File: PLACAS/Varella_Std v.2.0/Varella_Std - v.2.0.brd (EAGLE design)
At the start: 86 x 86 mm, 92 parts, among them IC1 74HC4051D,653, IC3 M95M04-DRDW6TP, IC4 M95M04-DRDW6TP, IC5 M95M04-DRDW6TP, IC6 M95M04-DRDW6TP, IC7 TESEO-LIV3F, IC8 BGA_725L6_E6327, U1 MAX31856, U2 MAX31856, U3 MAX31856, X1 JST-XH-02-PIN-ROUND-PAD, X2 JST-XH-02-PIN-ROUND-PAD, X3 JST-XH-02-PIN-ROUND-PAD

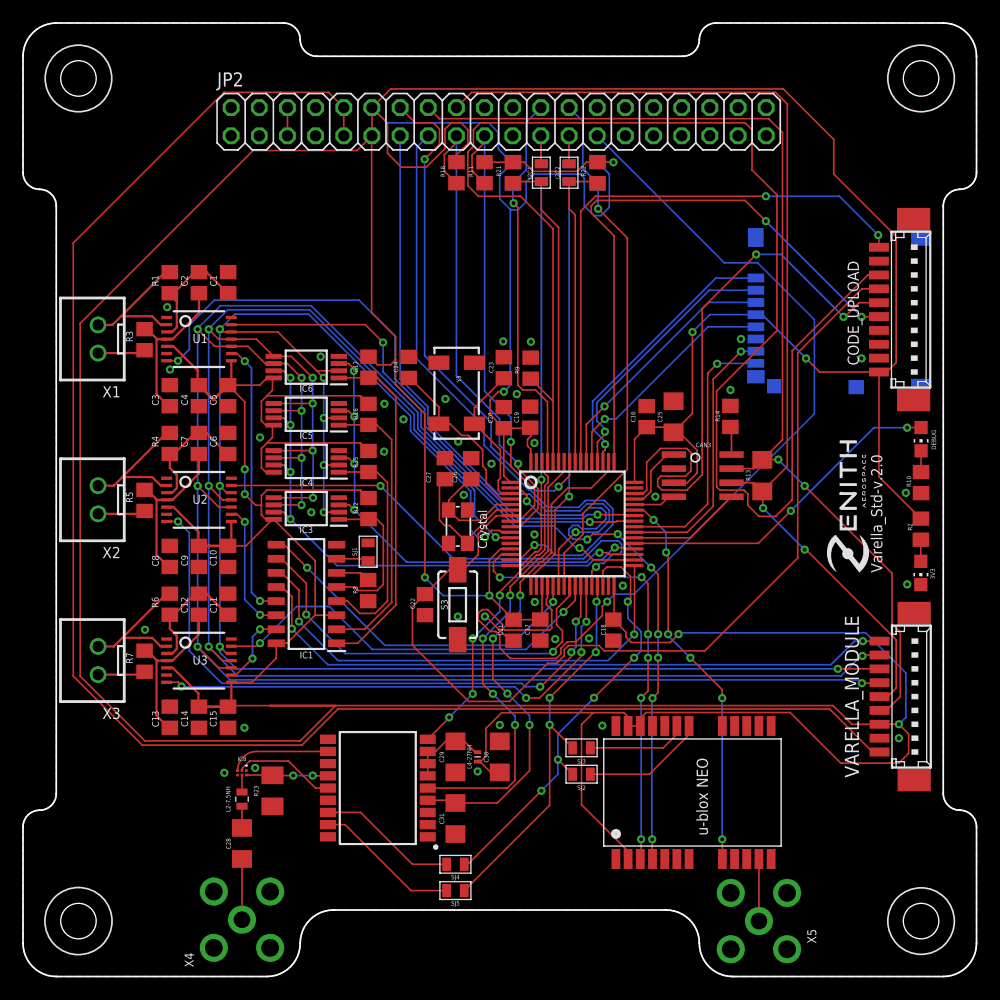
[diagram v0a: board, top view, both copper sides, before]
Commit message: Add files via upload
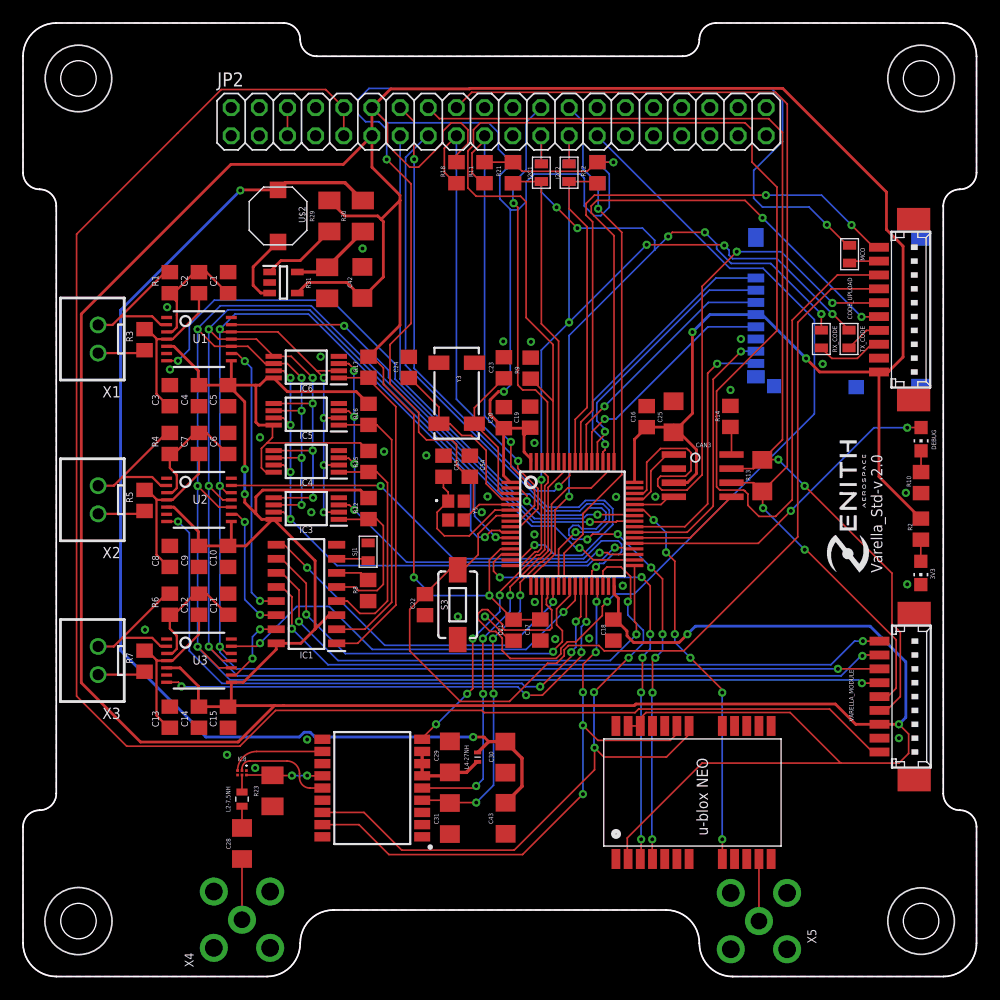
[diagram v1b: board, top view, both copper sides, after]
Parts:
- removed C26, C27: (no value), rcl:C0805
- removed SJ2, SJ3, SJ4, SJ5: (no value), FaBo-PIN:SMD-JUMPER-2
- removed U$7: CRYSTAL, cristal:CRYSTAL_SMD
- added C42: 56pF, rcl:C1206
- added C43: 22uF, rcl:C1206
- added C54, C55: 10pF, rcl:C0805
- added IC13: ST1S12GR, SamacSys_Parts:SOT95P280X110-5N
- added MCO, RX_CODE, TX_CODE: (no value), FaBo-PIN:SMD-JUMPER-2
- added R29: 1M, rcl (2):M1206
- added R30: 68k, rcl (2):M1206
- added R31: 27k, rcl (2):M1206
- added U$2: LTF5022T100M1R4, LTF5022T:LTF5022T
- added Y5: FA-20H_16.0000MF10Z-AJ0, SamacSys_Parts:FA20H160000MF12ZAC3
- C16, C17, C18, C19, C20: value (none) -> 100nF
- C21: value (none) -> 1uF
- C22: value (none) -> 0,1uF
- C23, C24: value (none) -> 10pF
- R10: value (none) -> 220
- R11, R12, R15, R16, R17, R18, R19, R20, R21, R22: value (none) -> 4,7k
- R8, R9: value (none) -> 1k
- moved C30 0.50 mm to (43.5, 19.8), turned to 270 degrees
- moved C29 0.50 mm to (38.5, 19.8), turned to 90 degrees
- moved C31 0.50 mm to (38.5, 14.2)
- moved IC7 0.50 mm to (31.5, 17.0)
- turned L4-27NH to 270 degrees
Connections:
- net SDA1/UART_TX renamed SDA1/UART_RX
- net SDA2/UART_RX renamed SDA2/UART_TX
- removed net SCL_NEOM8: SJ3.1, U$3.19
- removed net SCL_TESEO: IC7.17, SJ5.1
- removed net SDA_NEOM8: SJ2.1, U$3.18
- removed net SDA_TESEO: IC7.16, SJ4.1
- new net N$37: IC13.1, R29.1
- new net N$38: IC13.3, U$2.P$2
- new net N$39: IC13.5, R30.1, R31.2
- new net TESEO3: C30.1, C43.1, L4-27NH.1, R30.2, U$2.P$1
- new net UART_RX_CODE: CODE_UPLOAD.3, RX_CODE.2
- new net UART_TX_CODE: CODE_UPLOAD.4, TX_CODE.2
- net +3V3: now also C42.1, IC13.4, R29.2; no longer C30.1, L4-27NH.1
- net GND: now also C42.2, C43.2, C54.2, C55.2, IC13.2, R31.1, Y5.2, Y5.4; no longer C26.2, C27.2, U$7.P$1, U$7.P$4
- net MCO: now also MCO.2
- net OSC_IN: now also C54.1, MCO.1, Y5.3; no longer C26.1, U$7.P$2
- net OSC_OUT: now also C55.1, Y5.1; no longer C27.1, U$7.P$3
- net SCL4: now also IC7.17, U$3.19; no longer SJ3.2, SJ5.2
- net SDA4: now also IC7.16, U$3.18; no longer SJ2.2, SJ4.2
- net UART_RX: now also RX_CODE.1, UART_TX.2; no longer UART_RX.2
- net UART_TX: now also TX_CODE.1, UART_RX.2; no longer UART_TX.2
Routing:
- net TESEO3: track 0.00 -> 104.7 mm, vias 0 -> 2
- net OSC_IN: track 11.2 -> 110.4 mm, vias 0 -> 2
- net UART_TX: track 36.5 -> 69.1 mm, vias 1 -> 5
- net UART_RX: track 38.0 -> 69.3 mm, vias 1 -> 6
- net SDA4: track 39.6 -> 64.6 mm, vias 5 -> 4
- net SCL4: track 36.1 -> 57.7 mm, vias 4 -> 5
- net SCL_TESEO: track 13.2 -> 0.00 mm
- net SDA_TESEO: track 12.6 -> 0.00 mm
- net +3V3: track 683.8 -> 695.6 mm
- net SDA_NEOM8: track 11.2 -> 0.00 mm
- net SCL_NEOM8: track 9.08 -> 0.00 mm
- net N$39: track 0.00 -> 7.55 mm
- net N$37: track 0.00 -> 6.90 mm
- net N$38: track 0.00 -> 6.61 mm
- net UART_RX_CODE: track 0.00 -> 6.12 mm
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
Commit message: Add files via upload
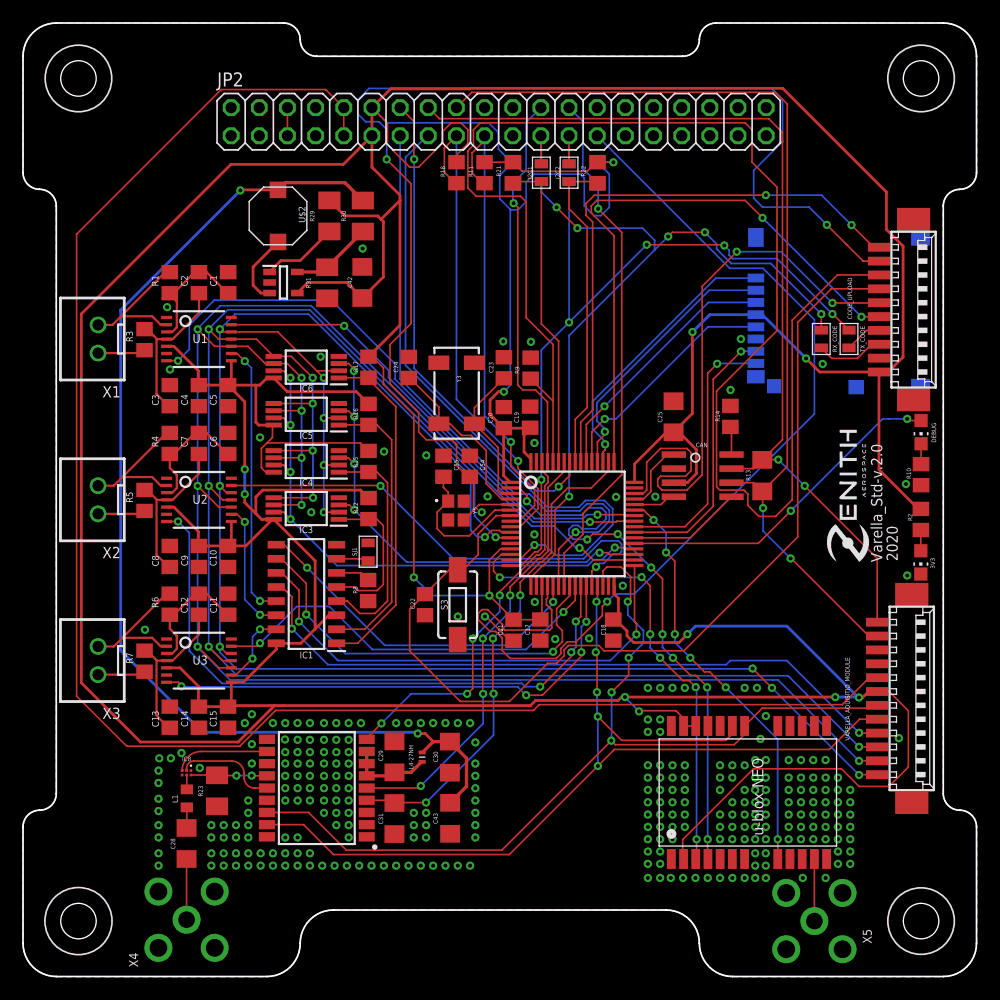
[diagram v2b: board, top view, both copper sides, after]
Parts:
- removed C16: 100nF, rcl:C0805
- removed L2-7,5NH: 0603CS-7N5XGLU, SamacSys_Parts:0603CS82NXGLW
- removed MCO: (no value), FaBo-PIN:SMD-JUMPER-2
- removed VARELLA_MODULE: 53398-09, con-molex:53398-09
- added L1: LQW18AS7N5J0ZD-7,5nH, LQW18AS7N5J0ZD:INDC1608X100N
- added VARELLA_AQUISITIO_MODULE: 53261-12, con-molex:53261-12
- CODE_UPLOAD: value 53398-10 -> 53261-10; device con-molex:53398-10 -> con-molex:53261-10
- moved C28 5.00 mm to (14.8, 12.0)
- moved C29 5.00 mm to (33.5, 19.8)
- moved C30 5.00 mm to (38.5, 19.8)
- moved C31 5.00 mm to (33.5, 14.2)
- moved C43 5.00 mm to (38.5, 14.3)
- moved IC7 5.00 mm to (26.5, 17.0)
- moved IC8 5.00 mm to (14.8, 18.4)
- moved L4-27NH 5.00 mm to (36.0, 19.8)
- moved R23 5.00 mm to (17.5, 16.8)
- moved U$3 5.00 mm to (65.9, 17.0)
- moved X4 5.00 mm to (14.8, 5.12)
- moved X5 5.00 mm to (71.4, 5.00)
- moved 3V3 0.95 mm to (81.0, 37.4)
- moved R2 0.87 mm to (81.0, 41.2)
- moved R10 0.71 mm to (81.0, 45.3)
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- renumbered CAN3 to CAN, COMM_MICRO1 to COMM_MICRO
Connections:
- net N$2 renamed L3
- removed net MCO: CODE_UPLOAD.9, MCO.2
- net +3V3: now also VARELLA_AQUISITIO_MODULE.7; no longer C16.1, VARELLA_MODULE.3
- net +5V: now also VARELLA_AQUISITIO_MODULE.8; no longer VARELLA_MODULE.1
- net CAN_H: now also VARELLA_AQUISITIO_MODULE.12; no longer VARELLA_MODULE.4
- net CAN_L: now also VARELLA_AQUISITIO_MODULE.11; no longer VARELLA_MODULE.5
- net GND: now also VARELLA_AQUISITIO_MODULE.10, VARELLA_AQUISITIO_MODULE.9; no longer C16.2, VARELLA_MODULE.2
- net MISO_SENSOR: now also VARELLA_AQUISITIO_MODULE.1; no longer VARELLA_MODULE.7
- net MOSI_SENSOR: now also VARELLA_AQUISITIO_MODULE.3; no longer VARELLA_MODULE.8
- net N$18: now also L1.2; no longer L2-7,5NH.2
- net N$19: now also L1.1; no longer L2-7,5NH.1
- net OSC_IN: now also CODE_UPLOAD.9; no longer MCO.1
- net SCL4: now also VARELLA_AQUISITIO_MODULE.5
- net SCLK_SENSOR: now also VARELLA_AQUISITIO_MODULE.2; no longer VARELLA_MODULE.6
- net SDA4: now also VARELLA_AQUISITIO_MODULE.6
- net Y3: now also VARELLA_AQUISITIO_MODULE.4; no longer VARELLA_MODULE.9
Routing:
- net SCL4: track 57.7 -> 93.0 mm
- net +3V3: track 695.6 -> 670.8 mm, vias 10 -> 13
- net SDA4: track 64.6 -> 84.5 mm
- net CAN_H: track 96.1 -> 86.1 mm
- net CAN_L: track 94.5 -> 87.7 mm
- net TESEO3: track 104.7 -> 99.3 mm
- net RESET_TESEO: track 30.2 -> 35.2 mm
- net MISO_SENSOR: track 159.5 -> 163.3 mm, vias 9 -> 11
- net OSC_IN: track 110.4 -> 113.6 mm
- net MCO: track 2.72 -> 0.00 mm
- net SCLK_SENSOR: track 179.3 -> 181.9 mm
- net RESET_NEOM8: track 35.2 -> 37.6 mm
- net PPS_TESEO: track 42.0 -> 44.4 mm
- net EXT_INTERRUPT_TESEO: track 37.6 -> 39.7 mm
- net PPS_NEOM8: track 42.3 -> 44.1 mm
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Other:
- board text added: "2020"

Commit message: Add files via upload
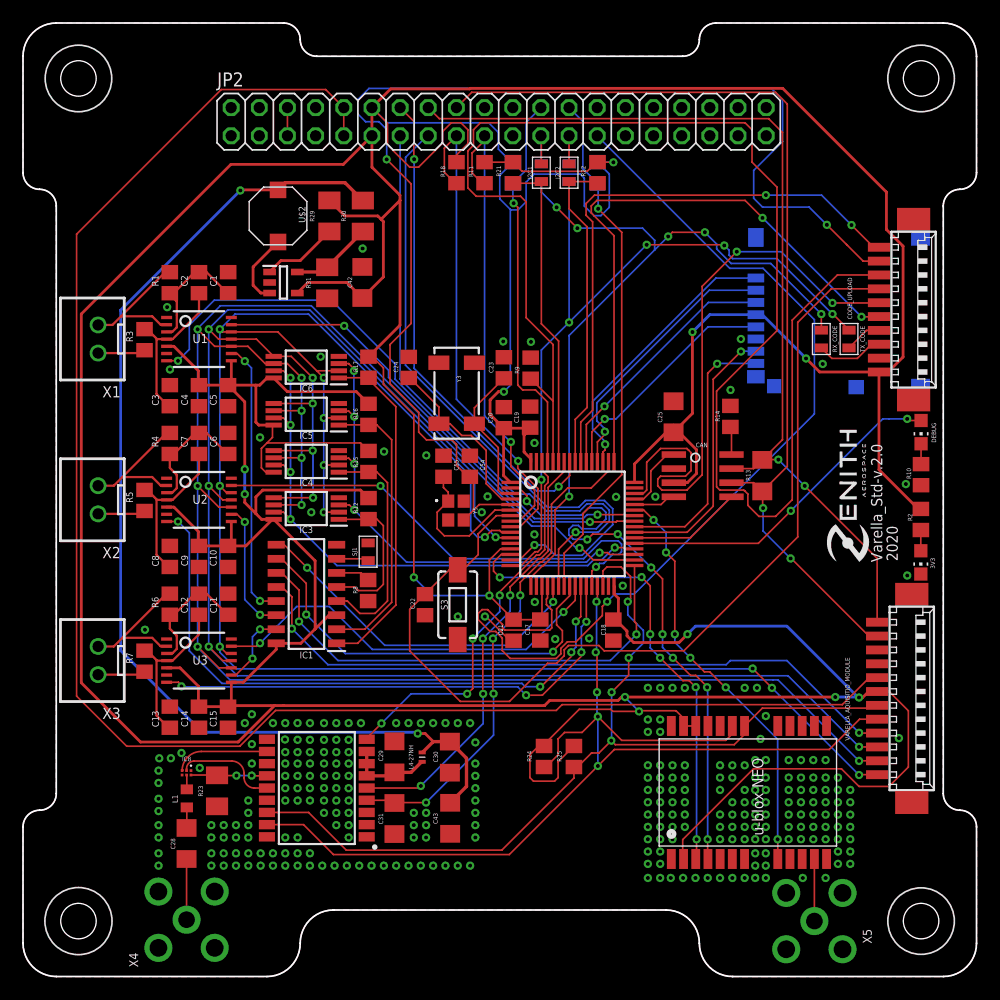
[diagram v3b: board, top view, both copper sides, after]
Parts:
- added R24, R25: 4,7k, rcl:R0805
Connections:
- net +3V3: now also R24.2, R25.2
- net SCL4: now also R24.1
- net SDA4: now also R25.1
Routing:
- net +3V3: track 670.8 -> 690.8 mm
- net SCL4: track 93.0 -> 100.6 mm
- net SDA4: track 84.5 -> 85.1 mm

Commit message: Add files via upload
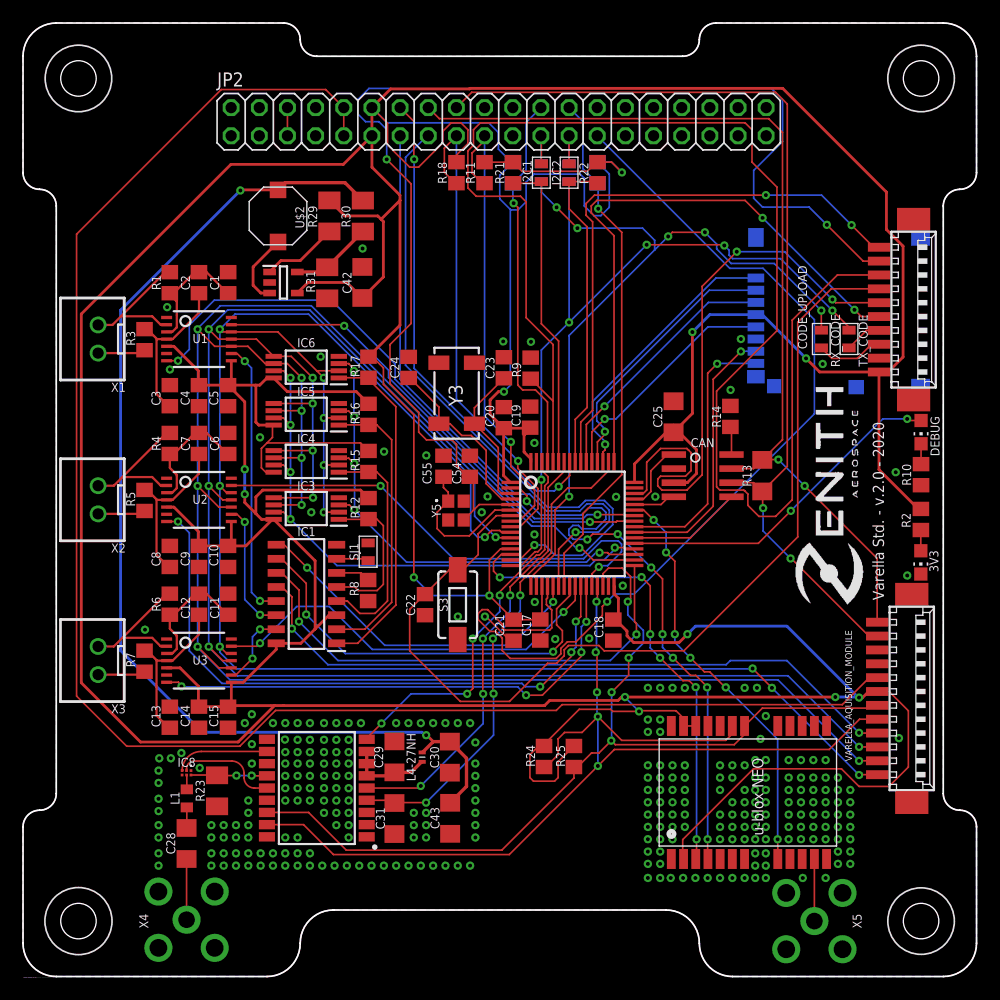
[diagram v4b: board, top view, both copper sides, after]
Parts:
- C30: value 1onF -> 10nF
- renumbered VARELLA_AQUISITIO_MODULE to VARELLA_AQUISITION_MODULE
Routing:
- net +3V3: track 690.8 -> 693.1 mm
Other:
- board text added: "C:/Users/marcu/Desktop/Ensino Superior/Graduação - Eng Elétrica/Zenith/zenith-v2.bmp"
- board text added: "C:/Users/marcu/Desktop/zenith-v3.bmp"
- board text added: "Varella Std. - v.2.0 - 2020"
- board text removed: "2020"
- board text removed: "Varella_Std-v.2.0"
